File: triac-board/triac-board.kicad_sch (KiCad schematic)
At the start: 24 parts, among them J1 Screw_Terminal_01x02, J2 Screw_Terminal_01x02, J3 Screw_Terminal_01x02, J4 Screw_Terminal_01x02, Q1 BTA16-600BW, Q2 BTA16-600BW, Q3 BTA16-600BW, Q4 BTA16-600BW, U1 MOC3063M, U2 MOC3063M, U3 MOC3063M, U4 MOC3063M

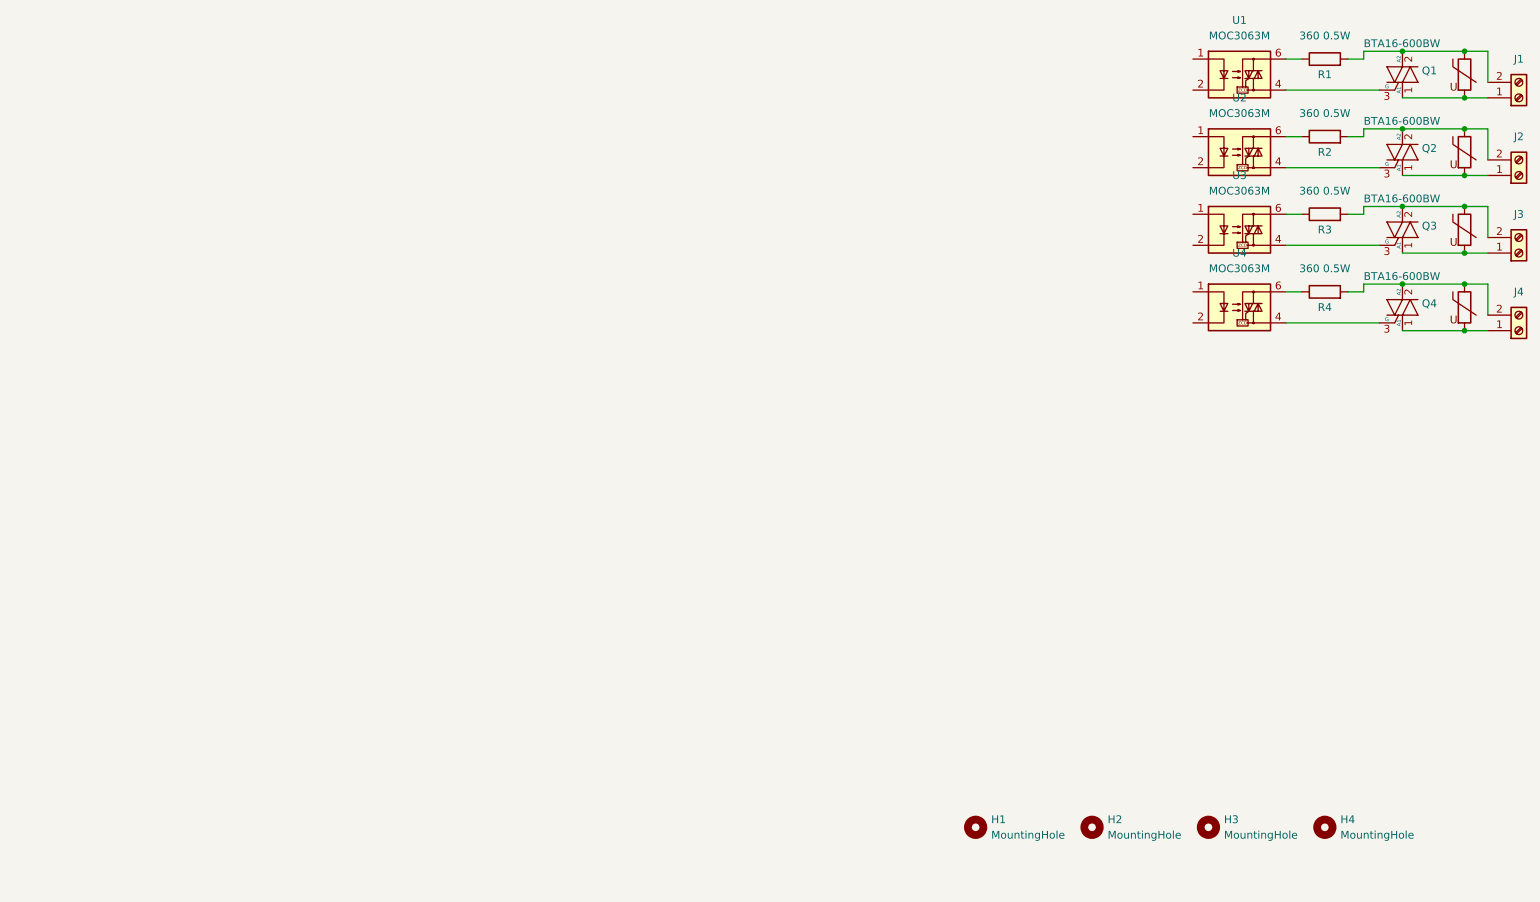
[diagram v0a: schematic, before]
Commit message: triac-board
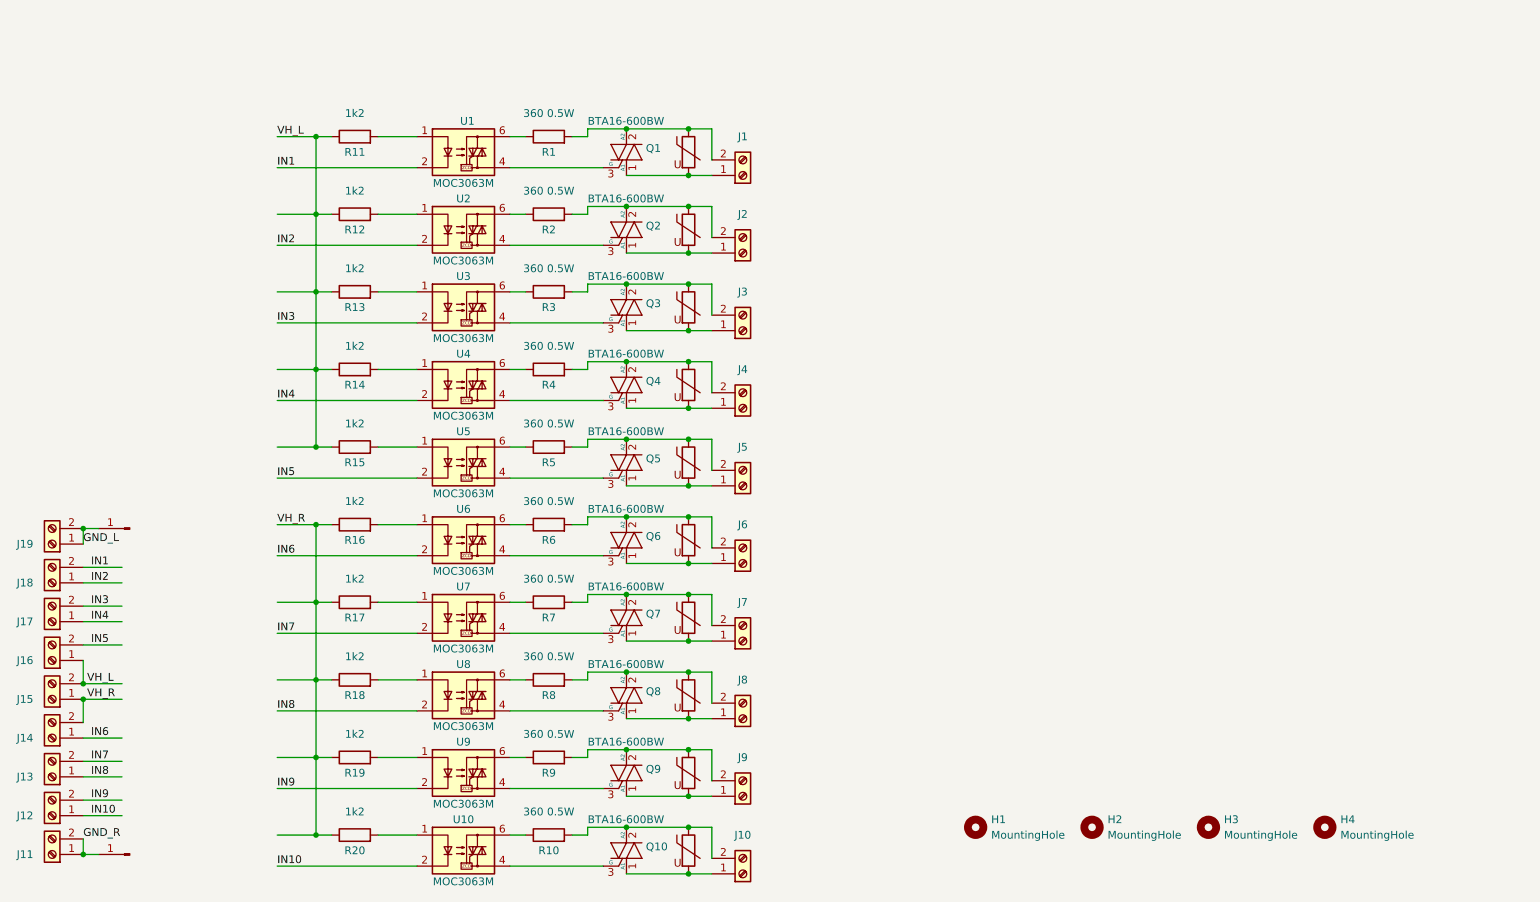
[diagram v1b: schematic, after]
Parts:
- added J10, J11, J12, J13, J14, J15, J16, J17, J18, J19, J5, J6, J7, J8, J9: Screw_Terminal_01x02, TerminalBlock_Phoenix:TerminalBlock_Phoenix_MKDS-1,5-2_1x02_P5.00mm_Horizontal, symbol Connector:Screw_Terminal_01x02
- added J20, J21: Conn_01x01_Male, Connector_Pin:Pin_D1.3mm_L11.0mm, symbol Connector:Conn_01x01_Male
- added Q10, Q5, Q6, Q7, Q8, Q9: BTA16-600BW, triac-board:TO-220-3_Vertical_Staggered, symbol Triac_Thyristor:BTA16-600BW
- added R10, R5, R6, R7, R8, R9: 360 0.5W, Resistor_THT:R_Axial_DIN0309_L9.0mm_D3.2mm_P20.32mm_Horizontal, symbol Device:R
- added R11, R12, R13, R14, R15, R16, R17, R18, R19, R20: 1k2, Resistor_THT:R_Axial_DIN0207_L6.3mm_D2.5mm_P10.16mm_Horizontal, symbol Device:R
- added RV10, RV5, RV6, RV7, RV8, RV9: 275V, Varistor:RV_Disc_D9mm_W4.2mm_P5mm, symbol Device:Varistor
- added U10, U5, U6, U7, U8, U9: MOC3063M, Package_DIP:DIP-6_W7.62mm, symbol Relay_SolidState:MOC3063M
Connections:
- net at U1.1: now also R11.2
- net IN1: now reaches U1.2
- net IN1: now also J18.2 (Pin_2)
- net at U2.1: now also R12.2
- net IN2: now reaches U2.2
- net IN2: now also J18.1 (Pin_1)
- net at U3.1: now also R13.2
- net IN3: now reaches U3.2
- net IN3: now also J17.2 (Pin_2)
- net at U4.1: now also R14.2
- net IN4: now reaches U4.2
- net IN4: now also J17.1 (Pin_1)
- new net: J7.2 (Pin_2), Q7.2 (A2), R7.2, RV7.1
- new net: J7.1 (Pin_1), Q7.1 (A1), RV7.2
- new net: R18.2, U8.1
- new net: Q8.3 (G), U8.4
- new net: R8.1, U8.6
- new net: J9.1 (Pin_1), Q9.1 (A1), RV9.2
- new net: J9.2 (Pin_2), Q9.2 (A2), R9.2, RV9.1
- new net: Q9.3 (G), U9.4
- new net: R5.1, U5.6
- new net: J5.2 (Pin_2), Q5.2 (A2), R5.2, RV5.1
- new net: R15.2, U5.1
- new net: Q7.3 (G), U7.4
- new net: J5.1 (Pin_1), Q5.1 (A1), RV5.2
- new net: R19.2, U9.1
- new net: R9.1, U9.6
- new net: J8.1 (Pin_1), Q8.1 (A1), RV8.2
- new net: J8.2 (Pin_2), Q8.2 (A2), R8.2, RV8.1
- new net: R16.2, U6.1
- new net: R20.2, U10.1
- new net: R7.1, U7.6
- new net: Q6.3 (G), U6.4
- new net: R6.1, U6.6
- new net: J6.1 (Pin_1), Q6.1 (A1), RV6.2
- new net: J6.2 (Pin_2), Q6.2 (A2), R6.2, RV6.1
- new net: J10.1 (Pin_1), Q10.1 (A1), RV10.2
- new net: J10.2 (Pin_2), Q10.2 (A2), R10.2, RV10.1
- new net: Q10.3 (G), U10.4
- new net: R10.1, U10.6
- new net: R17.2, U7.1
- new net: Q5.3 (G), U5.4
- new net GND_L: J19.1 (Pin_1), J19.2 (Pin_2), J20.1 (Pin_1)
- new net GND_R: J11.1 (Pin_1), J11.2 (Pin_2), J21.1 (Pin_1)
- new net IN10: J12.1 (Pin_1), U10.2
- new net IN5: J16.2 (Pin_2), U5.2
- new net IN6: J14.1 (Pin_1), U6.2
- new net IN7: J13.2 (Pin_2), U7.2
- new net IN8: J13.1 (Pin_1), U8.2
- new net IN9: J12.2 (Pin_2), U9.2
- new net VH_L: J15.2 (Pin_2), J16.1 (Pin_1), R11.1, R12.1, R13.1, R14.1, R15.1
- new net VH_R: J14.2 (Pin_2), J15.1 (Pin_1), R16.1, R17.1, R18.1, R19.1, R20.1
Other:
- moved on the sheet: J1, J2, J3, J4, Q1, Q2, Q3, Q4, R1, R2, R3, R4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
